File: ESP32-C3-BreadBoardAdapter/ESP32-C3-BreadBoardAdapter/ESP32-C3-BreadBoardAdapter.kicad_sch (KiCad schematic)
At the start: 2 parts, among them U1 ESP32-C3-WROOM-02-N4

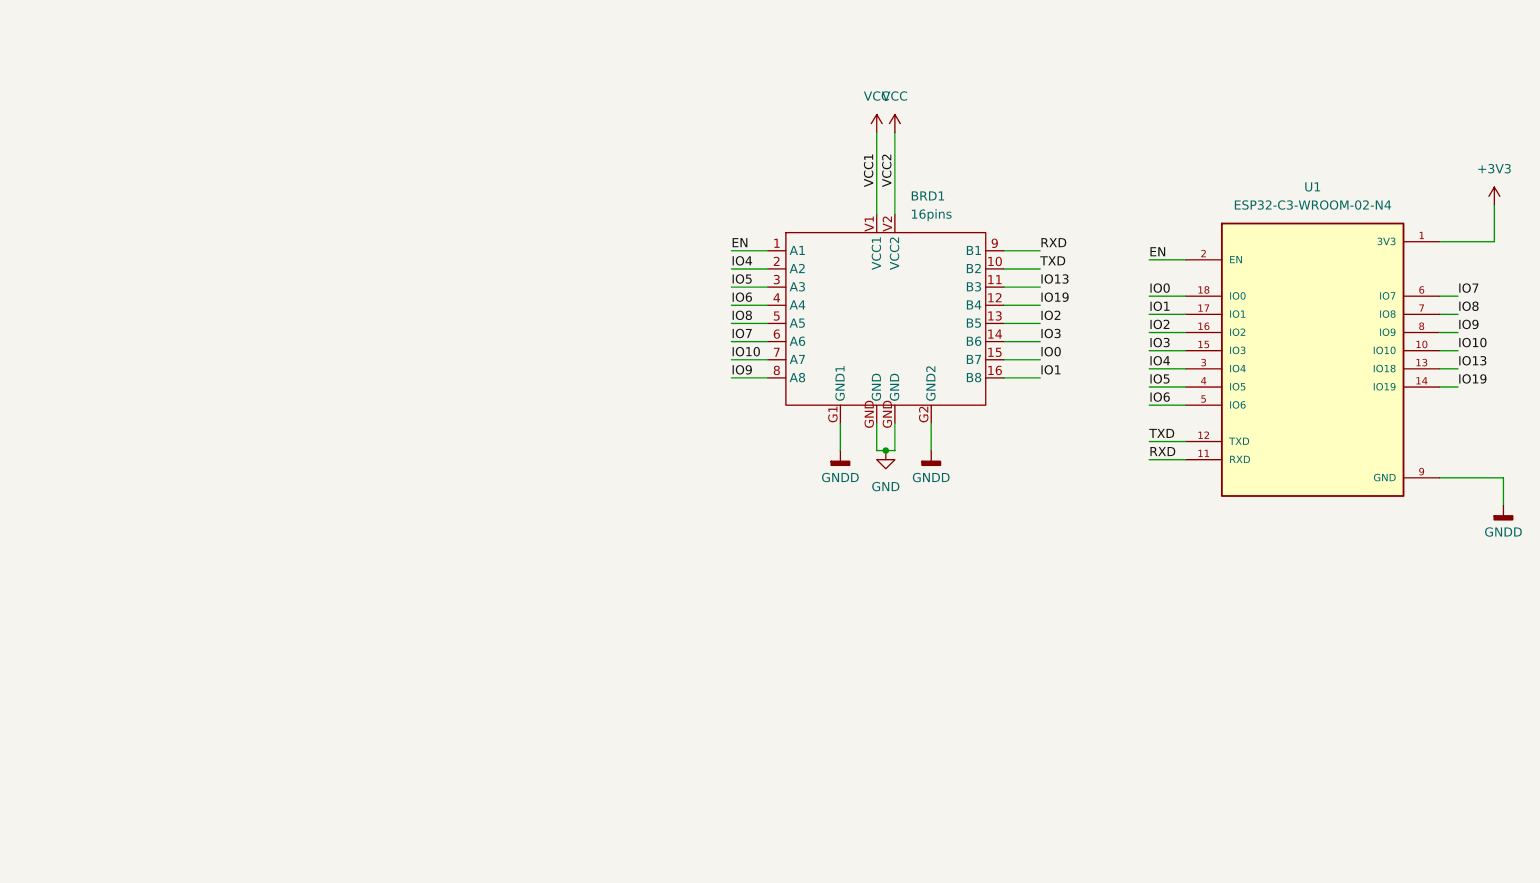
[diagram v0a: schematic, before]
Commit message: .
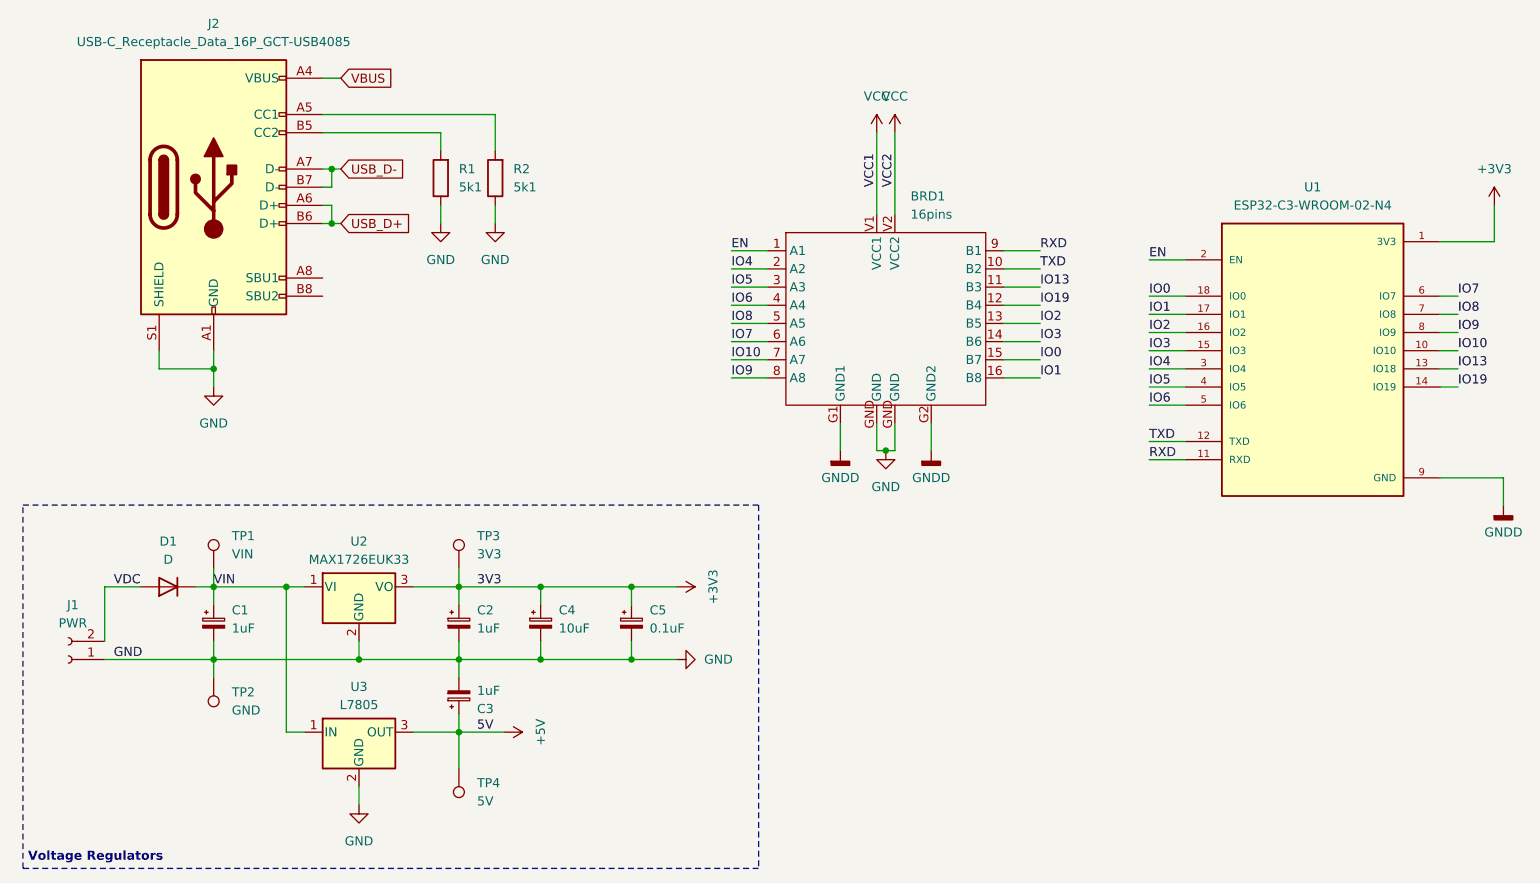
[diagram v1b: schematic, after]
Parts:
- added C1, C2, C3: 1uF, Capacitor_THT:CP_Radial_D4.0mm_P2.00mm, symbol Device:C_Polarized_Small
- added C4: 10uF, Capacitor_SMD:CP_Elec_3x5.3, symbol Device:C_Polarized_Small
- added C5: 0.1uF, Capacitor_SMD:CP_Elec_3x5.3, symbol Device:C_Polarized_Small
- added D1: D, Diode_SMD:D_1210_3225Metric, symbol Device:D
- added J1: PWR, Connector_PinSocket_2.54mm:PinSocket_1x02_P2.54mm_Vertical, symbol Connector:Conn_01x02_Socket
- added J2: USB-C_Receptacle_Data_16P_GCT-USB4085, Alexander Footprint Library:USB-C_GCT CONN16_USB4085-GF-A, symbol Alexander Symbol Library:USB-C_Receptacle_Data_16P_GCT-USB4085
- added R1, R2: 5k1, Resistor_SMD:R_1206_3216Metric_Pad1.30x1.75mm_HandSolder, symbol Device:R
- added TP1: VIN, TestPoint:TestPoint_Pad_D1.5mm, symbol Connector:TestPoint
- added TP2: GND, TestPoint:TestPoint_Pad_D1.5mm, symbol Connector:TestPoint
- added TP3: 3V3, TestPoint:TestPoint_Pad_D1.5mm, symbol Connector:TestPoint
- added TP4: 5V, TestPoint:TestPoint_Pad_D1.5mm, symbol Connector:TestPoint
- added U2: MAX1726EUK33, Package_TO_SOT_SMD:SOT-223-3_TabPin2, symbol Regulator_Linear:LM78M05_TO220
- added U3: L7805, Alexander Footprint Library:LD1117, symbol Regulator_Linear:L7805
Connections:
- net +3V3: now also C2.1, C4.1, C5.1, TP3.1, U2.3 (VO)
- net GND: now also C1.2, C2.2, C3.2, C4.2, C5.2, J1.1 (Pin_1), J2.A1 (GND), J2.A12 (GND), J2.B1 (GND), J2.B12 (GND), J2.S1 (SHIELD), J2.S2 (SHIELD), J2.S3 (SHIELD), J2.S4 (SHIELD), R1.1, R2.1, TP2.1, U2.2 (GND), U3.2 (GND)
- new net: J2.A5 (CC1), R2.2
- new net: J2.B5 (CC2), R1.2
- new net +5V: C3.1, TP4.1, U3.3 (OUT)
- new net USB_D+: J2.A6 (D+), J2.B6 (D+)
- new net USB_D-: J2.A7 (D-), J2.B7 (D-)
- new net VBUS: J2.A4 (VBUS), J2.A9 (VBUS), J2.B4 (VBUS), J2.B9 (VBUS)
- new net VDC: D1.2 (A), J1.2 (Pin_2)
- new net VIN: C1.1, D1.1 (K), TP1.1, U2.1 (VI), U3.1 (IN)
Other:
- note added: "Voltage Regulators"

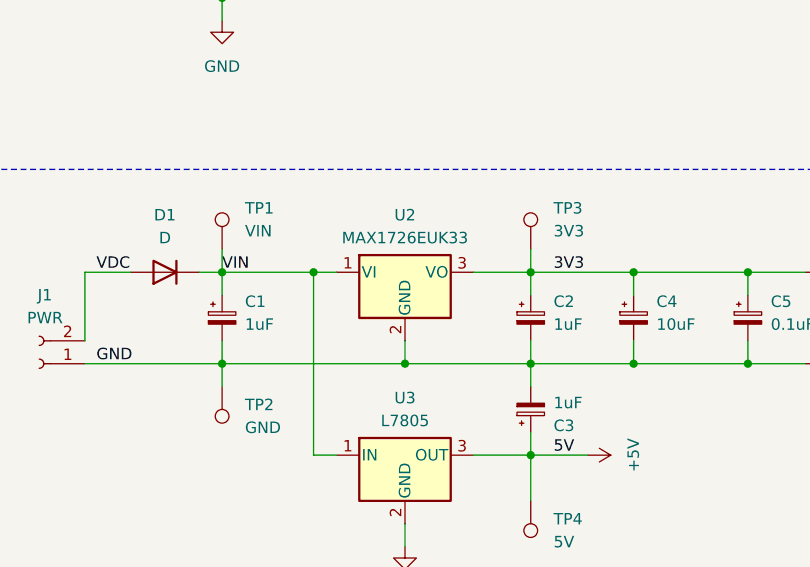
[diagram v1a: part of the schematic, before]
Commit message: .
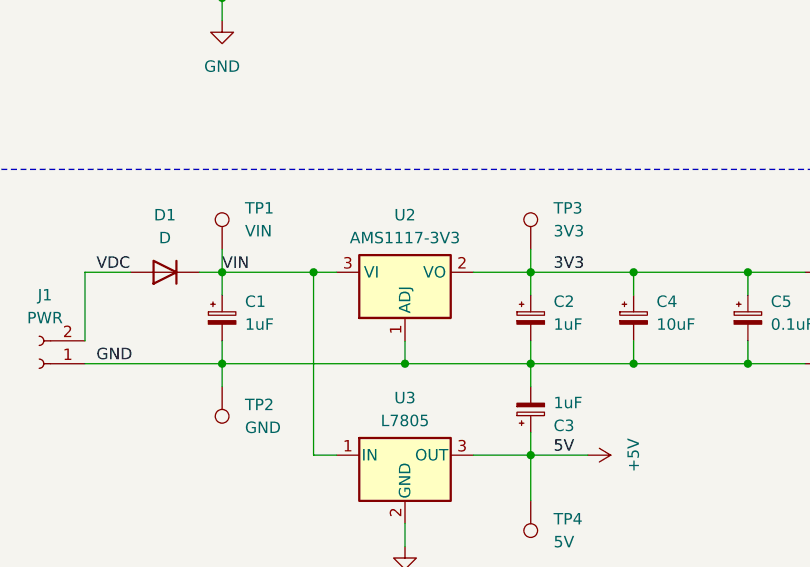
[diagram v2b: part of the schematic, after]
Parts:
- removed U2: MAX1726EUK33, Package_TO_SOT_SMD:SOT-223-3_TabPin2, symbol Regulator_Linear:LM78M05_TO220
- added U2: AMS1117-3V3, Alexander Footprint Library:AMS1117 SOT-223, symbol Alexander KiCad Libraries:AMS1117-3V3
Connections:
- net +3V3: now also U2.2 (VO)
- net GND: now also U2.1 (ADJ)
- net VIN: now also U2.3 (VI)
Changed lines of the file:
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@@
-	)
-	(symbol
-		(lib_id "Regulator_Linear:LM78M05_TO220")
-		(at 64.77 100.33 0)
-		(unit 1)
-		(exclude_from_sim no)
-		(in_bom yes)
-		(on_board yes)
-		(dnp no)
-		(property "Reference" "U2"
-			(at 64.77 93.98 0)
-			(effects
-				(font
-					(size 1.27 1.27)
-				)
-			)
-		)
-		(property "Value" "MAX1726EUK33"
-			(at 64.77 96.52 0)
-			(effects
-				(font
-					(size 1.27 1.27)
-				)
-			)
-		)
-		(property "Footprint" "Package_TO_SOT_SMD:SOT-223-3_TabPin2"
-			(at 64.77 94.615 0)
-			(effects
-				(font
-					(size 1.27 1.27)
-					(italic yes)
-				)
-				(hide yes)
-			)
-		)
-		(property "Datasheet" "https://www.onsemi.com/pub/Collateral/MC78M00-D.PDF"
-			(at 64.77 101.6 0)
-			(effects
-				(font
-					(size 1.27 1.27)
-				)
-				(hide yes)
-			)
-		)
-		(property "Description" ""
-			(at 64.77 100.33 0)
-			(effects
-				(font
-					(size 1.27 1.27)
-				)
-				(hide yes)
-			)
-		)
-		(pin "1"
-		)
-		(pin "2"
-		)
-		(pin "3"
-		)
-		(instances
-			(project "ESP32-C3-BreadBoardAdapter"
-				(path "/7ebe7346-feca-4308-bb7e-1ef2e739e742"
-					(reference "U2")
-					(unit 1)
-				)
-			)
-		)
 	)
 	(symbol
@@
 					(unit 1)
 				)
+			)
+		)
+	)
+	(symbol
+		(lib_id "Alexander KiCad Libraries:AMS1117-3V3")
+		(at 64.77 96.52 0)
+		(unit 1)
+		(exclude_from_sim yes)
+		(in_bom yes)
+		(on_board yes)
+		(dnp no)
+		(fields_autoplaced yes)
+		(property "Reference" "U2"
+			(at 64.77 93.98 0)
+			(effects
+				(font
+					(size 1.27 1.27)
+				)
+			)
+		)
+		(property "Value" "AMS1117-3V3"
+			(at 64.77 96.52 0)
+			(effects
+				(font
+					(size 1.27 1.27)
+				)
+			)
+		)
+		(property "Footprint" "Alexander Footprint Library:AMS1117 SOT-223"
+			(at 64.77 92.202 0)
+			(effects
+				(font
+					(size 1.27 1.27)
+				)
+				(hide yes)
+			)
+		)
+		(property "Datasheet" ""
+			(at 64.77 96.52 0)
+			(effects
+				(font
+					(size 1.27 1.27)
+				)
+				(hide yes)
+			)
+		)
+		(property "Description" "AMS1117"
+			(at 64.77 92.71 0)
+			(effects
+				(font
+					(size 1.27 1.27)
+				)
+				(hide yes)
+			)
+		)
+		(pin "2"
+		)
+		(pin "1"
+		)
+		(pin "3"
+		)
+		(instances
+			(project ""
+				(path "/7ebe7346-feca-4308-bb7e-1ef2e739e742"
+					(reference "U2")
+					(unit 1)
+				)
